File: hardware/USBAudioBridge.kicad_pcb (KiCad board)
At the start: 4 copper layers, 43.2 x 62 mm, 120 parts, among them J101 USB_C_Receptacle, J501 SWD, J502 UART, J601 PMOD_JB, J602 PMOD_JC, Q401 BSS84, SW301 RESET, SW401 BOOT, U1 MIMXRT1011DAE5A, U101 USBLC6-2SC6, U102 AP7361C-33E, U103 LP5907MFX-3.3, U301 MCP120T-300I/TT, U401 W25Q128JVSIQ, U601 CDCV304PW, X601 24.576MHz, Y301 24MHz, Y302 32.768kHz

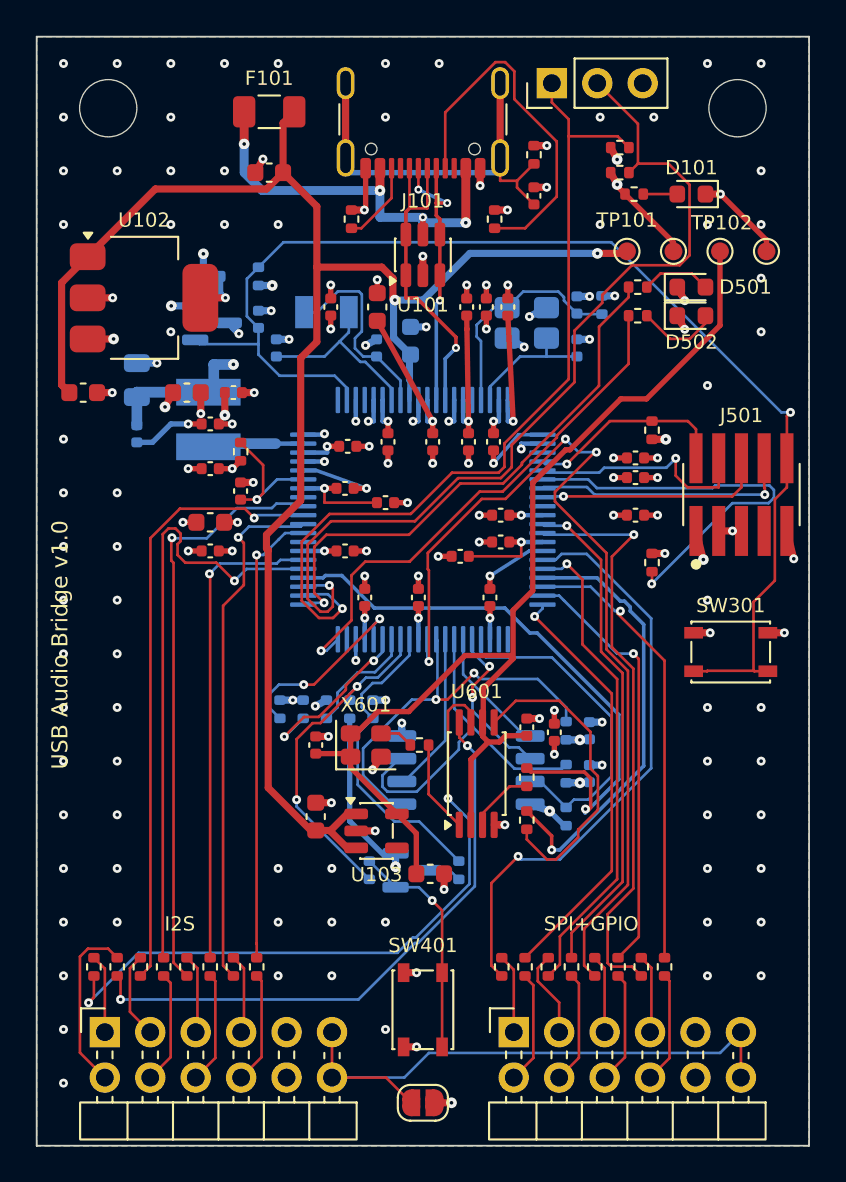
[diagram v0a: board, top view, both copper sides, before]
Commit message: improve manufacturability
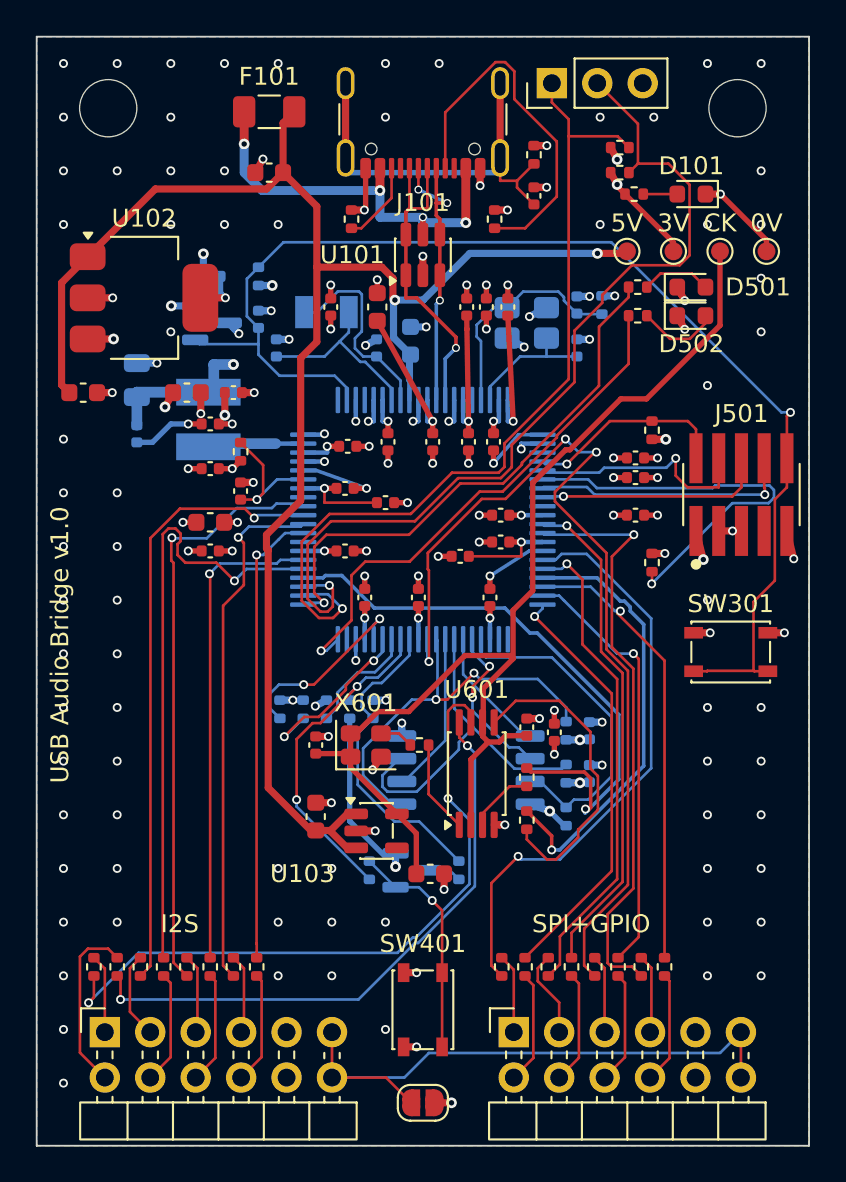
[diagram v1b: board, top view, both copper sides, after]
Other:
- board text added: "0V"
- board text added: "3V"
- board text added: "5V"
- board text added: "CK"
- board text added: "Hold BOOT, tap RESET: USB boot"
- board text removed: "Hold BOOT + tap RESET = USB serial downloader"
